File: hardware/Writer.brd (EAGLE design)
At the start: 68.6 x 53.3 mm, 20 parts, among them CN1 IRKit Wifi, IC1 JAPANINO-SLIM, SW1 SS12D01G4, SW2 SLIDE-SWITCH4/2

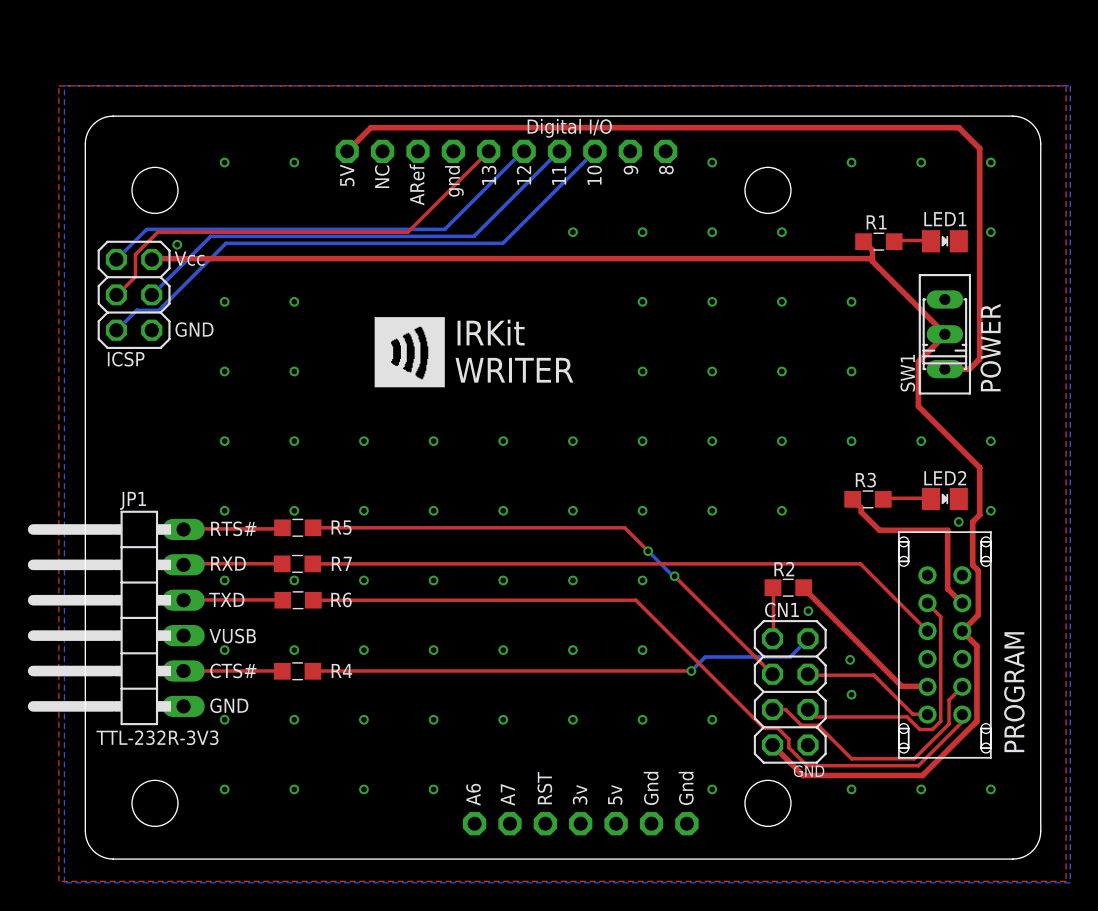
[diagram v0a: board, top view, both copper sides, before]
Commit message: looks fine
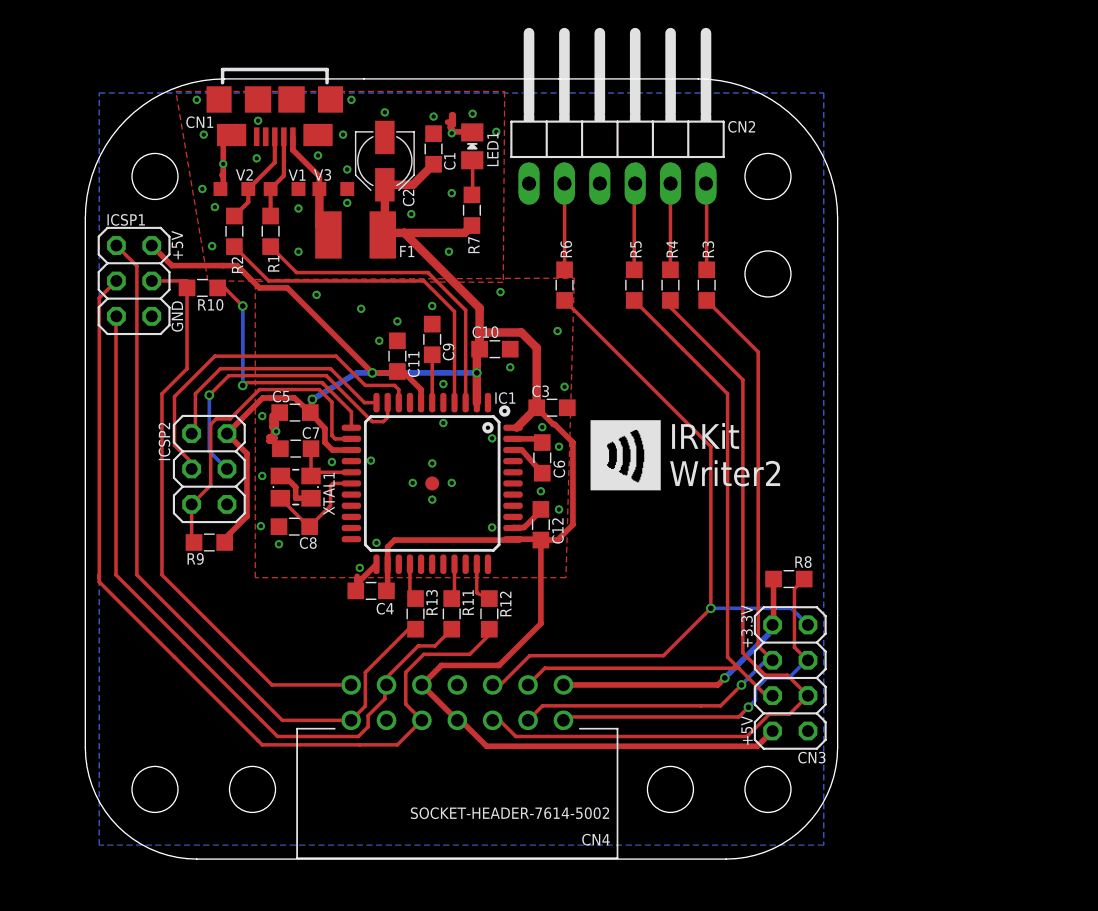
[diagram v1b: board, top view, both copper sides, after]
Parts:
- removed ICSP: IRKit ICSP, pinhead:2X03
- removed JP1: TTL-232R-3V3, pinhead:1X06/90
- removed LED2: OSG50805C1C, my:LED2012
- removed SW1: SS12D01G4, my:SS12D01G4
- removed SW2: SLIDE-SWITCH4/2, my:SLIDE-SWITCH-MCS421N
- added C1, C10, C11, C12, C3, C4, C5, C6: 0.1uF, my:SMD2012
- added C2: 10uF, my:PANASONIC_B
- added C7, C8: 12pF, my:SMD2012
- added C9: 1uF, my:SMD2012
- added CN2: TTL-232R-3V3, my:1X06/90
- added CN3: WiFi-Header, my:2X04
- added CN4: SOCKET-HEADER-7614-5002, my:SOCKET-HEADER-7614-5002
- added F1: MF-MSMF075-2, my:L1812
- added ICSP1: IRKit ICSP, my:2X03
- added ICSP2: Writer ICSP, my:2X03
- added R10, R11, R12, R13, R8: 1k, my:SMD2012
- added R9: 10k, my:SMD2012
- added SCREW1, SCREW2, SCREW3, SCREW4: flat-head M3 self-tapping, my:SCREW-M3
- added STANDOFF5, STANDOFF6, STANDOFF7: STAND-OFF, my:STAND-OFF
- added V1, V2, V3: CG0603MLC-05E, my:CT/CN0603
- added XTAL1: 16MHz CL:10pF, my:CRYSTAL-3.2-2.5
- CN1: value IRKit Wifi -> ZX62-B-5PA(11); device pinhead:2X04 -> my:USB-MICROB
- IC1: value JAPANINO-SLIM -> ATMEGA32U4AU; device my:JAPANINO-SLIM -> my:TQFP44-PAD
- R1: value 5.1k -> 22
- R2: value 1k -> 22
- R3: value 5.1k -> 1k
- R7: value 1k -> 5.1k
- moved STANDOFF1 61.5 mm to (49.0, 5.00)
- moved CN1 56.4 mm to (13.6, 54.5), turned to 180 degrees
- moved R2 47.3 mm to (10.7, 45.1), turned to 90 degrees
- moved STANDOFF4 45.0 mm to (5.00, 49.0)
- moved STANDOFF2 44.0 mm to (5.00, 5.00)
- moved R1 43.7 mm to (13.3, 45.1), turned to 90 degrees
- moved R4 38.5 mm to (42.0, 41.2), turned to 270 degrees
- moved IC1 36.7 mm to (24.9, 27.0), turned to 270 degrees
- moved LED1 34.6 mm to (27.8, 51.2), turned to 90 degrees
- moved R5 29.8 mm to (39.4, 41.2), turned to 270 degrees
- moved R6 29.6 mm to (34.4, 41.2), turned to 270 degrees
- moved R7 28.3 mm to (27.8, 46.6), turned to 90 degrees
- moved R3 19.3 mm to (44.6, 41.2), turned to 270 degrees
- moved U$1 17.2 mm to (36.3, 26.5)
- moved STANDOFF3 1.00 mm to (49.0, 49.0)
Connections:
- removed net 3V: IC1.3V
- removed net 5V: IC1.5V
- removed net MISO: IC1.D12, ICSP.1
- removed net MOSI: IC1.D11, ICSP.4
- removed net N$1: R6.1, SW2.1
- removed net N$10: R7.1, SW2.7
- removed net N$2: R3.1, SW2.C2
- removed net N$4: R2.1, SW2.C3
- removed net N$5: SW2.8
- removed net N$6: LED2.A, R3.2
- removed net N$7: SW2.2
- removed net N$8: SW1.3
- removed net N$9: SW2.6
- removed net RESET: IC1.D10, ICSP.5
- removed net SCK: IC1.D13, ICSP.3
- removed net VCC: CN1.7, ICSP.2, R1.1, SW1.2, SW2.3
- removed net VEXT: IC1.5V@2, SW1.1
- new net +5V: C1.1, C10.2, C11.2, C12.2, C2.+, C3.2, C4.2, C5.2, CN3.7, CN4.10, CN4.7, F1.2, IC1.14, IC1.2, IC1.24, IC1.34, IC1.44, IC1.7, ICSP1.2, ICSP2.2, R7.1, R9.2
- new net A0: IC1.36
- new net A1: IC1.37
- new net A2: IC1.38
- new net A3: IC1.39
- new net A4: IC1.40
- new net A5: IC1.41
- new net AREF: C6.2, IC1.42
- new net D0: IC1.20
- new net D1: IC1.21
- new net D10: IC1.30, R11.1
- new net D11: IC1.12, R10.1
- new net D12: IC1.26, R13.1
- new net D13: IC1.32, R12.1
- new net D2: IC1.19
- new net D3: IC1.18
- new net D4: IC1.25
- new net D5: IC1.31
- new net D6: IC1.27
- new net D7: IC1.1
- new net D8: IC1.28
- new net D9: IC1.29
- new net HWB: IC1.33
- new net IRKIT/!RESET: CN4.12, ICSP1.5, R11.2
- new net IRKIT/MISO: CN4.13, ICSP1.1, R13.2
- new net IRKIT/MOSI: CN4.14, ICSP1.4, R10.2
- new net IRKIT/SCK: CN4.9, ICSP1.3, R12.2
- new net N$48: CN1.P2, R1.2, V1.1
- new net N$51: CN1.P3, R2.2, V2.1
- new net N$52: CN1.P1, F1.1, V3.1
- new net RXLED: IC1.8
- new net TXLED: IC1.22
- new net UCAP: C9.2, IC1.6
- new net USB+: IC1.4, R2.1
- new net USB-: IC1.3, R1.1
- new net USB-ID: CN1.P4
- new net WRITER/!RESET: IC1.13, ICSP2.5, R9.1
- new net WRITER/MISO: IC1.11, ICSP2.1
- new net WRITER/MOSI: IC1.10, ICSP2.4
- new net WRITER/SCK: IC1.9, ICSP2.3
- new net XTAL1: C8.2, IC1.17, XTAL1.1
- new net XTAL2: C7.2, IC1.16, XTAL1.3
- net +3V3: now also CN3.1, CN4.2, R8.2; no longer CN1.1, R2.2
- net CTS#: now also CN2.2, R6.1; no longer JP1.2, R4.2
- net GND: now also C1.2, C10.1, C11.1, C12.1, C2.-, C3.1, C4.1, C5.1, C6.1, C7.1, C8.1, C9.1, CN1.P5, CN1.S1, CN1.S2, CN1.S3, CN1.S4, CN1.S5, CN1.S6, CN2.1, CN3.8, CN4.11, CN4.8, IC1.15, IC1.23, IC1.35, IC1.43, IC1.5, IC1.P$1, ICSP1.6, ICSP2.6, V1.2, V2.2, V3.2, XTAL1.2, XTAL1.4; no longer CN1.8, IC1.GND, IC1.GND1, IC1.GND2, ICSP.6, JP1.1, LED2.K, SW2.4
- net N$3: now also R7.2; no longer R1.2
- net RTS#: now also CN2.6, R3.1; no longer JP1.6, R5.2
- net RXD: now also CN2.5, R4.1; no longer JP1.5, R7.2
- net TXD: now also CN2.4, R5.1; no longer JP1.4, R6.2
- net VUSB: now also CN2.3; no longer JP1.3
- net WIFI_UART0_CTS: now also CN3.3, CN4.3, R3.2; no longer CN1.3, R5.1
- net WIFI_UART0_RTS: now also CN3.2, CN4.6, R6.2; no longer CN1.2, R4.1
- net WIFI_UART0_RX: now also CN3.5, CN4.4, R5.2; no longer CN1.5, SW2.C1
- net WIFI_UART0_TX: now also CN3.6, CN4.5, R4.2; no longer CN1.6, SW2.C4
- net WIFI_UART1_RTS: now also CN3.4, CN4.1, R8.1; no longer CN1.4, SW2.5
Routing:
- net +5V: track 0.00 -> 171.8 mm, vias 0 -> 3
- net VCC: track 109.7 -> 0.00 mm
- net VEXT: track 64.6 -> 0.00 mm
- net IRKIT/SCK: track 0.00 -> 63.3 mm
- net N$1: track 53.7 -> 0.00 mm
- net IRKIT/MISO: track 0.00 -> 52.7 mm
- net IRKIT/!RESET: track 0.00 -> 52.0 mm
- net N$10: track 46.1 -> 0.00 mm
- net IRKIT/MOSI: track 0.00 -> 41.9 mm
- net RESET: track 39.7 -> 0.00 mm
- net WIFI_UART0_TX: track 19.5 -> 57.7 mm
- net MOSI: track 33.5 -> 0.00 mm
- net MISO: track 32.5 -> 0.00 mm
- net SCK: track 31.9 -> 0.00 mm
- net WIFI_UART0_RX: track 18.2 -> 48.4 mm
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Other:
- board size 68.6 x 53.3 mm -> 54 x 56 mm
- board text added: "+3.3V"
- board text added: "+5V"
- board text added: "IRKit Writer2"
- board text removed: "CTS#"
- board text removed: "IRKit WRITER"
- board text removed: "POWER"
- board text removed: "PROGRAM"
- board text removed: "RTS#"
- board text removed: "RXD"
- board text removed: "TTL-232R-3V3"
- board text removed: "TXD"
- board text removed: "VUSB"
- board text removed: "Vcc"
